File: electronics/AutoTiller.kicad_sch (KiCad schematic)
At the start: 96 parts, among them IC1 ESP32-C3-MINI-1-N4, J1 USB_C_Receptacle_USB2.0, J3 UART, SW1 Reset, SW2 +1, SW2 +15, SW2 -1, SW2 -15, SW2 L, SW2 R, SW5 Power

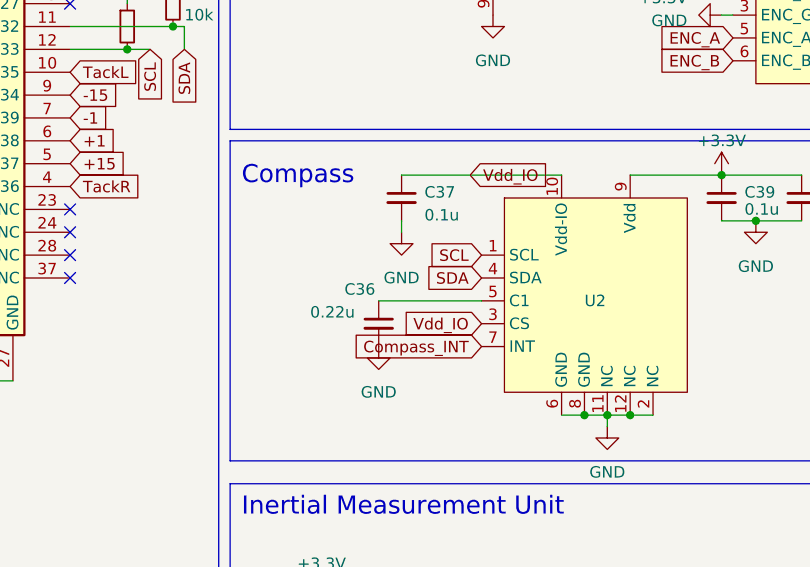
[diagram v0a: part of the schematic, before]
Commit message: MVP
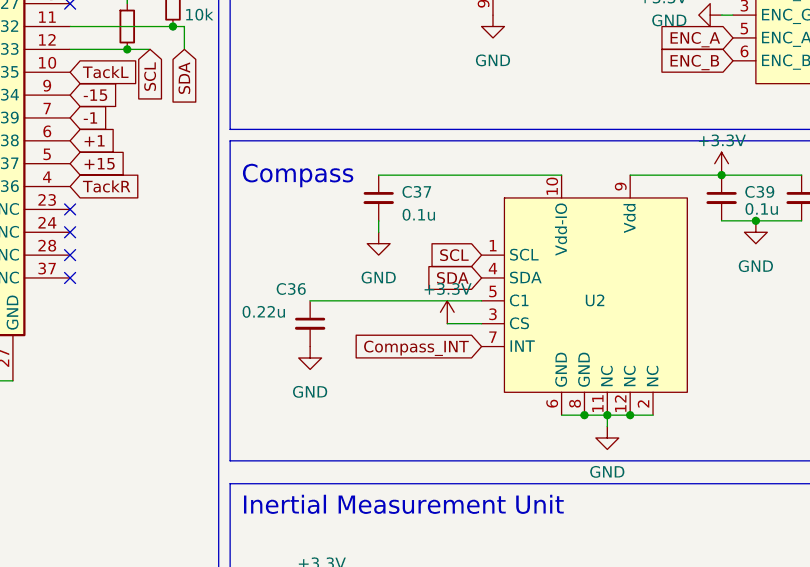
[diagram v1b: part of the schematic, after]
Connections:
- net +3.3V: now also U2.3 (CS)
- net Vdd_IO: no longer names the net of C37.1, U2.10 (Vdd-IO)
- net Vdd_IO: no longer U2.3 (CS)
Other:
- moved on the sheet: C36, C37
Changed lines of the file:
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@@
     (stroke (width 0) (type default))
   )
-  (wire (pts (xy 222.25 72.39) (xy 222.25 73.66))
+  (wire (pts (xy 219.71 72.39) (xy 219.71 73.66))
     (stroke (width 0) (type default))
   )
@@
     (stroke (width 0) (type default))
   )
-  (wire (pts (xy 219.71 81.28) (xy 231.14 81.28))
+  (wire (pts (xy 212.09 81.28) (xy 231.14 81.28))
     (stroke (width 0) (type default))
   )
@@
     (stroke (width 0) (type default))
   )
-  (wire (pts (xy 222.25 67.31) (xy 240.03 67.31))
+  (wire (pts (xy 219.71 67.31) (xy 240.03 67.31))
     (stroke (width 0) (type default))
   )
@@
     (stroke (width 0) (type default))
   )
+  (wire (pts (xy 231.14 83.82) (xy 227.33 83.82))
+    (stroke (width 0) (type default))
+  )
   (wire (pts (xy 166.37 90.17) (xy 168.91 90.17))
     (stroke (width 0) (type default))
@@
     )
   )
-  (global_label "Vdd_IO" (shape input) (at 231.14 83.82 180) (fields_autoplaced)
-    (effects (font (size 1.27 1.27)) (justify right))
-    (property "Intersheetrefs" "${INTERSHEET_REFS}" (at 221.9447 83.82 0)
-      (effects (font (size 1.27 1.27)) (justify right) hide)
-    )
-  )
   (global_label "REGN" (shape input) (at 144.78 168.91 90) (fields_autoplaced)
     (effects (font (size 1.27 1.27)) (justify left))
@@
     )
   )
-  (global_label "Vdd_IO" (shape input) (at 229.87 67.31 0) (fields_autoplaced)
-    (effects (font (size 1.27 1.27)) (justify left))
-    (property "Intersheetrefs" "${INTERSHEET_REFS}" (at 239.0653 67.31 0)
-      (effects (font (size 1.27 1.27)) (justify left) hide)
-    )
-  )
   (global_label "D-" (shape input) (at 80.01 172.72 0) (fields_autoplaced)
     (effects (font (size 1.27 1.27)) (justify left))
@@
     )
   )
-  (symbol (lib_id "Device:C_Small") (at 219.71 83.82 0) (unit 1)
+  (symbol (lib_id "Device:C_Small") (at 212.09 83.82 0) (unit 1)
     (in_bom yes) (on_board yes) (dnp no)
-    (property "Reference" "C36" (at 215.9 80.01 0)
+    (property "Reference" "C36" (at 208.28 80.01 0)
       (effects (font (size 1.27 1.27)) (justify left))
     )
-    (property "Value" "0.22u" (at 212.09 82.55 0)
+    (property "Value" "0.22u" (at 204.47 82.55 0)
       (effects (font (size 1.27 1.27)) (justify left))
     )
-    (property "Footprint" "Capacitor_SMD:C_0402_1005Metric" (at 219.71 83.82 0)
+    (property "Footprint" "Capacitor_SMD:C_0402_1005Metric" (at 212.09 83.82 0)
       (effects (font (size 1.27 1.27)) hide)
     )
-    (property "Datasheet" "~" (at 219.71 83.82 0)
+    (property "Datasheet" "~" (at 212.09 83.82 0)
       (effects (font (size 1.27 1.27)) hide)
     )
@@
     )
   )
-  (symbol (lib_id "power:GND") (at 222.25 73.66 0) (unit 1)
+  (symbol (lib_id "power:GND") (at 219.71 73.66 0) (unit 1)
     (in_bom yes) (on_board yes) (dnp no) (fields_autoplaced)
-    (property "Reference" "#PWR057" (at 222.25 80.01 0)
+    (property "Reference" "#PWR057" (at 219.71 80.01 0)
       (effects (font (size 1.27 1.27)) hide)
     )
-    (property "Value" "GND" (at 222.25 78.74 0)
+    (property "Value" "GND" (at 219.71 78.74 0)
       (effects (font (size 1.27 1.27)))
     )
-    (property "Footprint" "" (at 222.25 73.66 0)
+    (property "Footprint" "" (at 219.71 73.66 0)
       (effects (font (size 1.27 1.27)) hide)
     )
-    (property "Datasheet" "" (at 222.25 73.66 0)
+    (property "Datasheet" "" (at 219.71 73.66 0)
       (effects (font (size 1.27 1.27)) hide)
     )
@@
     )
   )
-  (symbol (lib_id "power:GND") (at 219.71 86.36 0) (unit 1)
+  (symbol (lib_id "power:GND") (at 212.09 86.36 0) (unit 1)
     (in_bom yes) (on_board yes) (dnp no) (fields_autoplaced)
-    (property "Reference" "#PWR055" (at 219.71 92.71 0)
+    (property "Reference" "#PWR055" (at 212.09 92.71 0)
       (effects (font (size 1.27 1.27)) hide)
     )
-    (property "Value" "GND" (at 219.71 91.44 0)
+    (property "Value" "GND" (at 212.09 91.44 0)
       (effects (font (size 1.27 1.27)))
     )
-    (property "Footprint" "" (at 219.71 86.36 0)
+    (property "Footprint" "" (at 212.09 86.36 0)
       (effects (font (size 1.27 1.27)) hide)
     )
-    (property "Datasheet" "" (at 219.71 86.36 0)
+    (property "Datasheet" "" (at 212.09 86.36 0)
       (effects (font (size 1.27 1.27)) hide)
     )
@@
     )
   )
-  (symbol (lib_id "Device:C_Small") (at 222.25 69.85 0) (unit 1)
+  (symbol (lib_id "Device:C_Small") (at 219.71 69.85 0) (unit 1)
     (in_bom yes) (on_board yes) (dnp no) (fields_autoplaced)
-    (property "Reference" "C37" (at 224.79 69.2213 0)
+    (property "Reference" "C37" (at 222.25 69.2213 0)
       (effects (font (size 1.27 1.27)) (justify left))
     )
-    (property "Value" "0.1u" (at 224.79 71.7613 0)
+    (property "Value" "0.1u" (at 222.25 71.7613 0)
       (effects (font (size 1.27 1.27)) (justify left))
     )
-    (property "Footprint" "Capacitor_SMD:C_0402_1005Metric" (at 222.25 69.85 0)
+    (property "Footprint" "Capacitor_SMD:C_0402_1005Metric" (at 219.71 69.85 0)
       (effects (font (size 1.27 1.27)) hide)
     )
-    (property "Datasheet" "~" (at 222.25 69.85 0)
+    (property "Datasheet" "~" (at 219.71 69.85 0)
       (effects (font (size 1.27 1.27)) hide)
     )
@@
         )
       )
+    )
+  )
+  (symbol (lib_id "power:+3.3V") (at 227.33 83.82 0) (unit 1)
+    (in_bom yes) (on_board yes) (dnp no) (fields_autoplaced)
+    (property "Reference" "#PWR062" (at 227.33 87.63 0)
+      (effects (font (size 1.27 1.27)) hide)
+    )
+    (property "Value" "+3.3V" (at 227.33 80.01 0)
+      (effects (font (size 1.27 1.27)))
+    )
+    (property "Footprint" "" (at 227.33 83.82 0)
+      (effects (font (size 1.27 1.27)) hide)
+    )
+    (property "Datasheet" "" (at 227.33 83.82 0)
+      (effects (font (size 1.27 1.27)) hide)
+    )
+    (pin "1")
+    (instances
+      (project "AutoTiller"
+        (path "/8fe1d5bf-4000-444d-9640-67eaa880ff39"
+          (reference "#PWR062") (unit 1)
+        )
+      )
